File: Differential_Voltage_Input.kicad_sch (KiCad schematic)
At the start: 5 parts, among them J5 DIFFERENTIAL VOLTAGE INPUT, U8 D3V3XA4B10LP

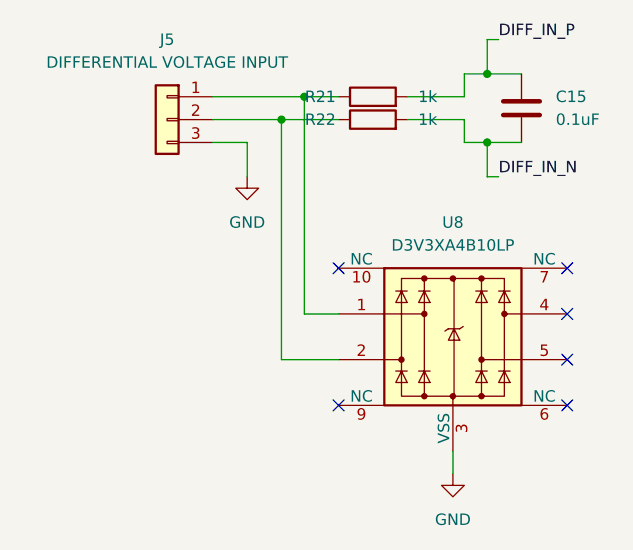
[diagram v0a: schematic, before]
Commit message: finished schematic draft 1
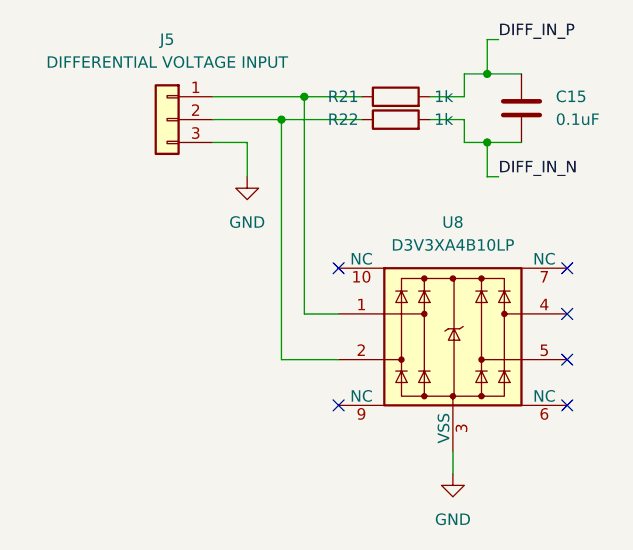
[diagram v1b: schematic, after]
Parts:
- J5: footprint Package_DFN_QFN:Diodes_UDFN-10_1x2.5mm_P0.5mm -> TerminalBlock_Phoenix:TerminalBlock_Phoenix_MKDS-1,5-3-5.08_1x03_P5.08mm_Horizontal; MPN (none) -> 1715734; Manufacturer (none) -> Phoenix Contact
- U8: MPN (none) -> D3V3XA4B10LP-7; Manufacturer (none) -> Diodes Incorporated
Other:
- moved on the sheet: R21, R22
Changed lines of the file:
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@@
 	(wire
 		(pts
-			(xy 83.82 82.55) (xy 90.17 82.55)
+			(xy 83.82 82.55) (xy 92.71 82.55)
 		)
 		(stroke
@@
 	(wire
 		(pts
-			(xy 97.79 80.01) (xy 104.14 80.01)
+			(xy 100.33 80.01) (xy 104.14 80.01)
 		)
 		(stroke
@@
 	(wire
 		(pts
-			(xy 86.36 80.01) (xy 90.17 80.01)
+			(xy 86.36 80.01) (xy 92.71 80.01)
 		)
 		(stroke
@@
 	(wire
 		(pts
-			(xy 97.79 82.55) (xy 104.14 82.55)
+			(xy 100.33 82.55) (xy 104.14 82.55)
 		)
 		(stroke
@@
 			)
 		)
-		(property "Footprint" "Package_DFN_QFN:Diodes_UDFN-10_1x2.5mm_P0.5mm"
+		(property "Footprint" "TerminalBlock_Phoenix:TerminalBlock_Phoenix_MKDS-1,5-3-5.08_1x03_P5.08mm_Horizontal"
 			(at 71.12 82.55 0)
 			(hide yes)
@@
 		)
 		(property "Description" "Generic connector, single row, 01x03, script generated (kicad-library-utils/schlib/autogen/connector/)"
+			(at 71.12 82.55 0)
+			(hide yes)
+			(show_name no)
+			(do_not_autoplace no)
+			(effects
+				(font
+					(size 1.27 1.27)
+				)
+			)
+		)
+		(property "Manufacturer" "Phoenix Contact"
+			(at 71.12 82.55 0)
+			(hide yes)
+			(show_name no)
+			(do_not_autoplace no)
+			(effects
+				(font
+					(size 1.27 1.27)
+				)
+			)
+		)
+		(property "MPN" "1715734"
 			(at 71.12 82.55 0)
 			(hide yes)
@@
 	(symbol
 		(lib_id "Device:R")
-		(at 93.98 82.55 90)
+		(at 96.52 82.55 90)
 		(unit 1)
 		(body_style 1)
@@
 		(dnp no)
 		(property "Reference" "R22"
-			(at 88.138 82.55 90)
+			(at 90.678 82.55 90)
 			(show_name no)
 			(do_not_autoplace no)
@@
 		)
 		(property "Value" "1k"
-			(at 100.076 82.55 90)
+			(at 101.854 82.55 90)
 			(show_name no)
 			(do_not_autoplace no)
@@
 		)
 		(property "Footprint" ""
-			(at 93.98 84.328 90)
+			(at 96.52 84.328 90)
 			(hide yes)
 			(show_name no)
@@
 		)
 		(property "Datasheet" ""
-			(at 93.98 82.55 0)
+			(at 96.52 82.55 0)
 			(hide yes)
 			(show_name no)
@@
 		)
 		(property "Description" "Resistor"
-			(at 93.98 82.55 0)
+			(at 96.52 82.55 0)
 			(hide yes)
 			(show_name no)
@@
 	(symbol
 		(lib_id "Device:R")
-		(at 93.98 80.01 90)
+		(at 96.52 80.01 90)
 		(unit 1)
 		(body_style 1)
@@
 		(dnp no)
 		(property "Reference" "R21"
-			(at 88.138 80.01 90)
+			(at 90.678 80.01 90)
 			(show_name no)
 			(do_not_autoplace no)
@@
 		)
 		(property "Value" "1k"
-			(at 100.076 80.01 90)
+			(at 101.854 80.01 90)
 			(show_name no)
 			(do_not_autoplace no)
@@
 		)
 		(property "Footprint" ""
-			(at 93.98 81.788 90)
+			(at 96.52 81.788 90)
 			(hide yes)
 			(show_name no)
@@
 		)
 		(property "Datasheet" ""
-			(at 93.98 80.01 0)
+			(at 96.52 80.01 0)
 			(hide yes)
 			(show_name no)
@@
 		)
 		(property "Description" "Resistor"
-			(at 93.98 80.01 0)
+			(at 96.52 80.01 0)
 			(hide yes)
 			(show_name no)
@@
 			(at 102.87 106.68 0)
 			(hide yes)
+			(show_name no)
+			(do_not_autoplace no)
+			(effects
+				(font
+					(size 1.27 1.27)
+				)
+			)
+		)
+		(property "Manufacturer" "Diodes Incorporated"
+			(at 102.87 106.68 0)
+			(hide yes)
+			(show_name no)
+			(do_not_autoplace no)
+			(effects
+				(font
+					(size 1.27 1.27)
+				)
+			)
+		)
+		(property "MPN" "D3V3XA4B10LP-7"
+			(at 102.87 106.68 0)
+			(hide yes)
